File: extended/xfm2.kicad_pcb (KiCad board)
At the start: 2 copper layers, 69.2 x 121.3 mm, 32 parts, among them J1 Midi In, J2 Pin Breakout, J3 Midi Out, J4 Midi Thru, J5 Conn_Coaxial, U1 H11L1, U2 CmodA7-35T, U3 24LC01, U4 UDA1334A, U5 74HC14

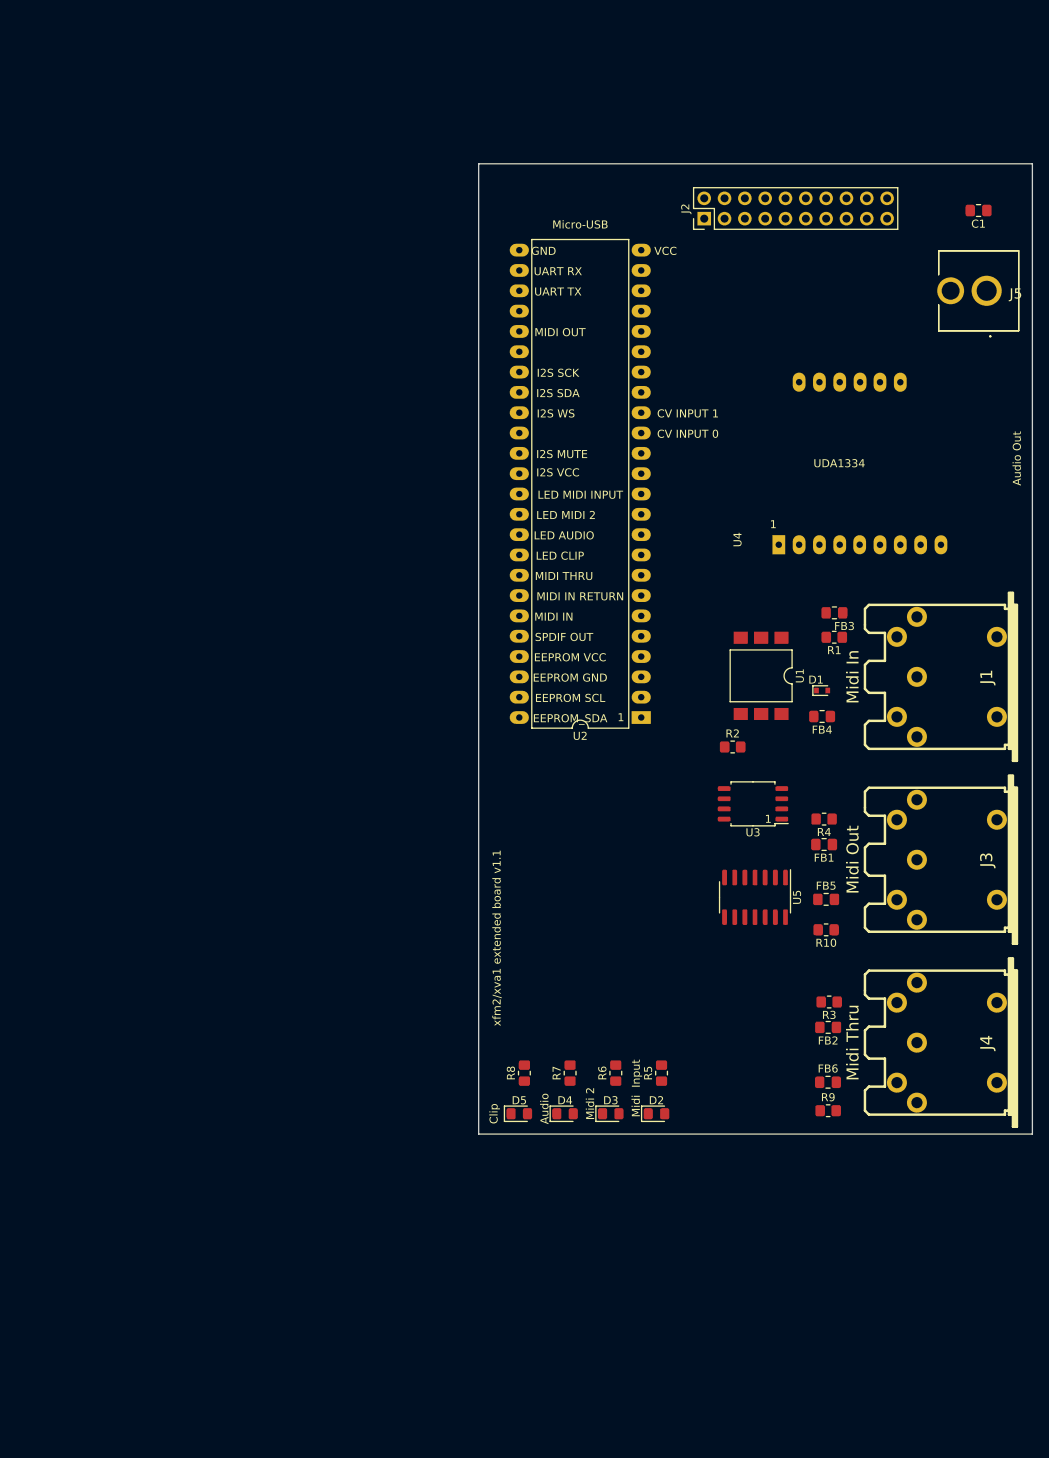
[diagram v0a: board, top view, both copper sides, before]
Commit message: initial extended pcb 1.1 placement
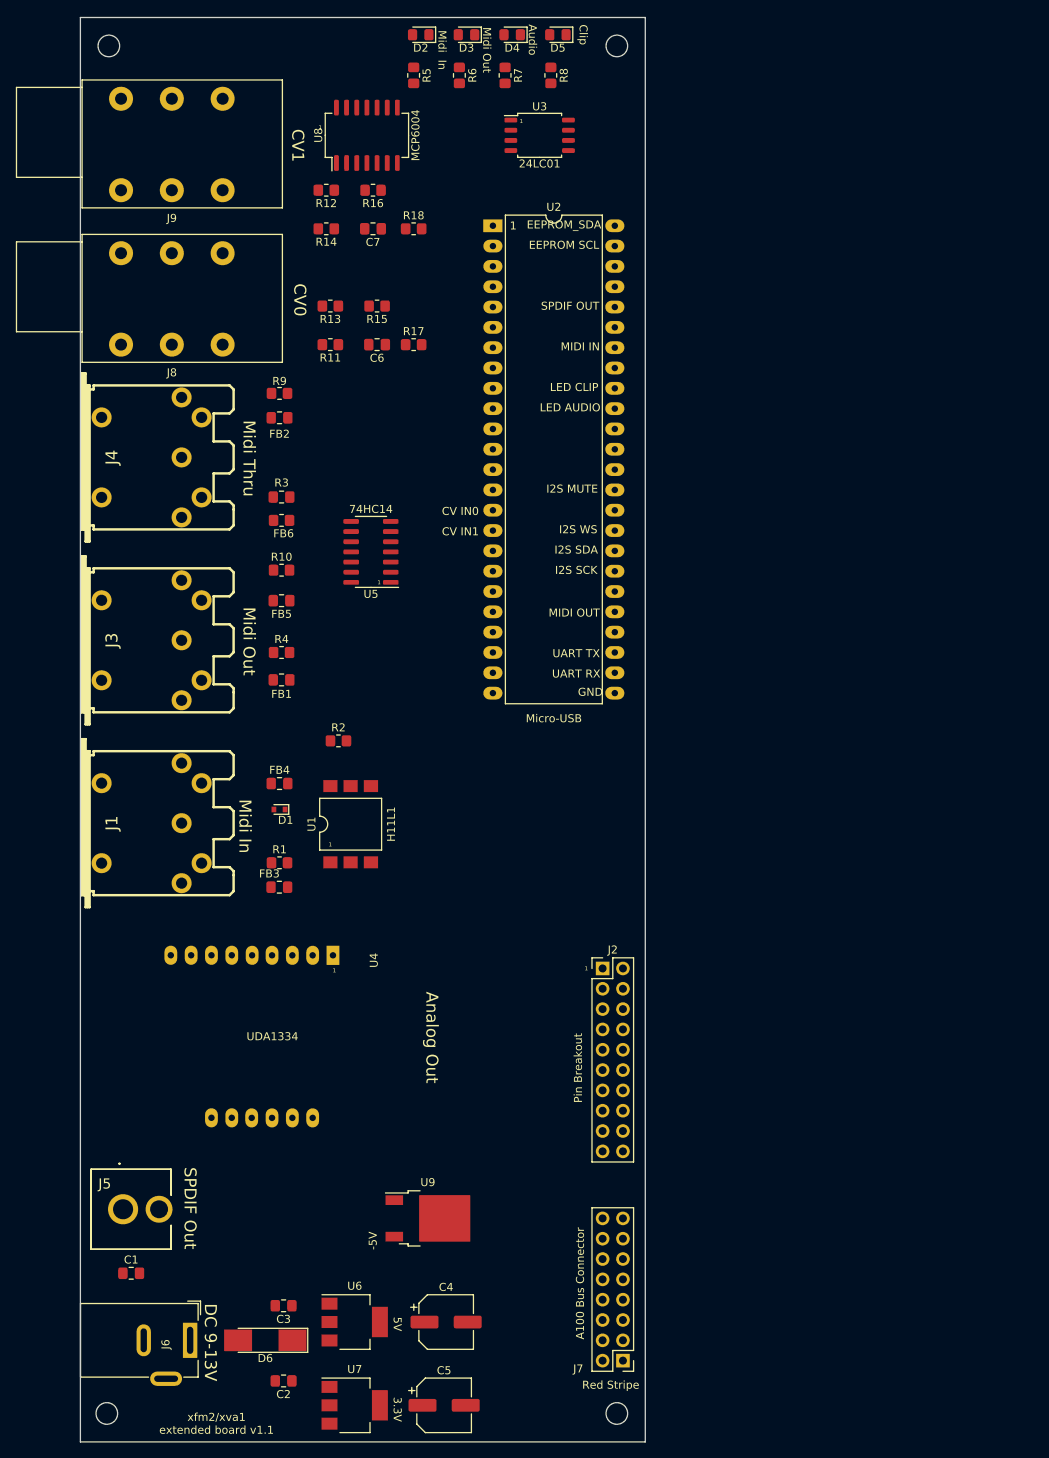
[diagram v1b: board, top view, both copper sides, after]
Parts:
- added C2: 10uF, Capacitor_SMD:C_0805_2012Metric_Pad1.18x1.45mm_HandSolder, F.Cu at (111.5, 186.4)
- added C3: 10uF, Capacitor_SMD:C_0805_2012Metric_Pad1.18x1.45mm_HandSolder, F.Cu at (111.5, 177.0)
- added C4: 100uF, Capacitor_SMD:CP_Elec_6.3x5.7, F.Cu at (131.8, 179.1)
- added C5: 100uF, Capacitor_SMD:CP_Elec_6.3x5.7, F.Cu at (131.6, 189.5)
- added C6: 330p-560p, Capacitor_SMD:C_0805_2012Metric_Pad1.18x1.45mm_HandSolder, F.Cu at (123.2, 56.9)
- added C7: 330p-560p, Capacitor_SMD:C_0805_2012Metric_Pad1.18x1.45mm_HandSolder, F.Cu at (122.7, 42.4)
- added D6: 1N4007, Diode_SMD:D_MELF_Handsoldering, F.Cu at (109.2, 181.4)
- added J6: Jack-DC, Connector_BarrelJack:BarrelJack_Wuerth_6941xx301002, F.Cu at (99.8, 181.4)
- added J7: A-100_Bus_Connector, Connector_PinHeader_2.54mm:PinHeader_2x08_P2.54mm_Vertical, F.Cu at (153.9, 183.9)
- added J8: AudioJack2, Connector_Audio:Jack_6.35mm_Neutrik_NRJ6HM-1_Horizontal, F.Cu at (103.9, 56.9)
- added J9: AudioJack2, Connector_Audio:Jack_6.35mm_Neutrik_NRJ6HM-1_Horizontal, F.Cu at (103.9, 37.6)
- added R11: 100k, Resistor_SMD:R_0805_2012Metric_Pad1.20x1.40mm_HandSolder, F.Cu at (117.3, 56.9)
- added R12: 100k, Resistor_SMD:R_0805_2012Metric_Pad1.20x1.40mm_HandSolder, F.Cu at (116.8, 37.6)
- added R13: 100k, Resistor_SMD:R_0805_2012Metric_Pad1.20x1.40mm_HandSolder, F.Cu at (117.3, 52.1)
- added R14: 100k, Resistor_SMD:R_0805_2012Metric_Pad1.20x1.40mm_HandSolder, F.Cu at (116.8, 42.4)
- added R15: 33k, Resistor_SMD:R_0805_2012Metric_Pad1.20x1.40mm_HandSolder, F.Cu at (123.2, 52.1)
- added R16: 33k, Resistor_SMD:R_0805_2012Metric_Pad1.20x1.40mm_HandSolder, F.Cu at (122.7, 37.6)
- added R17: 100, Resistor_SMD:R_0805_2012Metric_Pad1.20x1.40mm_HandSolder, F.Cu at (127.8, 56.9)
- added R18: 100, Resistor_SMD:R_0805_2012Metric_Pad1.20x1.40mm_HandSolder, F.Cu at (127.8, 42.4)
- added REF**: , MountingHole:MountingHole_2.7mm_M2.5, F.Cu at (89.7, 19.6)
- added REF**: , MountingHole:MountingHole_2.7mm_M2.5, F.Cu at (153.2, 19.6)
- added REF**: , MountingHole:MountingHole_2.7mm_M2.5, F.Cu at (153.2, 190.5)
- added REF**: , MountingHole:MountingHole_2.7mm_M2.5, F.Cu at (89.4, 190.5)
- added U6: LM1117-5.0, Package_TO_SOT_SMD:SOT-223-3_TabPin2, F.Cu at (120.4, 179.1)
- added U7: LM1117-3.3, Package_TO_SOT_SMD:SOT-223-3_TabPin2, F.Cu at (120.4, 189.5)
- added U8: MCP6004, Package_SO:SO-14_5.3x10.2mm_P1.27mm, F.Cu at (121.9, 30.7)
- added U9: MC79M05_TO252, Package_TO_SOT_SMD:TO-252-2, F.Cu at (129.5, 166.1)
- moved C1 169.9 mm to (92.5, 173.0), turned to 0 degrees
- moved J5 157.6 mm to (91.4, 165.0), turned to 0 degrees
- moved D2 138.1 mm to (128.7, 18.2), turned to 180 degrees
- moved D3 136.1 mm to (134.4, 18.2), turned to 180 degrees
- moved D4 135.0 mm to (140.1, 18.2), turned to 180 degrees
- moved D5 135.0 mm to (145.8, 18.2), turned to 180 degrees
- moved R5 128.5 mm to (127.8, 23.2), turned to 270 degrees
- moved R6 126.2 mm to (133.5, 23.2), turned to 270 degrees
- moved R7 125.0 mm to (139.2, 23.2), turned to 270 degrees
- moved R8 124.8 mm to (144.9, 23.2), turned to 270 degrees
- moved J4 122.2 mm to (95.8, 71.0), turned to 270 degrees
- moved R9 112.9 mm to (111.0, 63.0), turned to 180 degrees
- moved FB2 102.5 mm to (111.0, 66.0), turned to 0 degrees
- moved J3 101.7 mm to (95.8, 93.9), turned to 270 degrees
- moved FB6 100.1 mm to (111.3, 75.9), turned to 180 degrees
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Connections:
- J2 pad 10: I2S_VCC -> Net-(J2-Pad10)
- J2 pad 18: Net-(J2-Pad18) -> -5V
- J2 pad 19: Net-(J2-Pad19) -> +5V
- J2 pad 20: VCC -> +3V3
- R2 pad 1: EEPROM_VCC -> +3V3
- R3 pad 1: I2S_VCC -> +3V3
- R4 pad 2: I2S_VCC -> +3V3
- U1 pad 6: I2S_VCC -> +3V3
- U2 pad 15: Net-(U2-Pad15) -> CV0_3.3V
- U2 pad 16: Net-(U2-Pad16) -> CV1_3.3V
- U2 pad 24: VCC -> +5V
- U2 pad 36: I2S_VCC -> Net-(U2-Pad36)
- U2 pad 45: EEPROM_VCC -> Net-(U2-Pad45)
- U3 pad 3: EEPROM_VCC -> +3V3
- U3 pad 8: EEPROM_VCC -> +3V3
- U4 pad 1: I2S_VCC -> +3V3
- U4 pad 11: I2S_VCC -> +3V3
- U4 pad 13: I2S_VCC -> +3V3
- U5 pad 14: I2S_VCC -> +3V3
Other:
- board size 69.2 x 121.3 mm -> 70.6 x 178.1 mm
- board text added: "-5V"
- board text added: "24LC01"
- board text added: "3.3V"
- board text added: "5V"
- board text added: "74HC14"
- board text added: "A100 Bus Connector"
- board text added: "Analog Out"
- board text added: "CV IN0"
- board text added: "CV IN1"
- board text added: "CV0"
- board text added: "CV1"
- board text added: "DC 9-13V"
- board text added: "H11L1"
- board text added: "MCP6004"
- board text added: "Midi In"
- board text added: "Midi Out"
- board text added: "Midi Thru"
- board text added: "Pin Breakout"
- board text added: "Red Stripe"
- board text added: "SPDIF Out"
- board text removed: "Audio Out"
- board text removed: "CV INPUT 0"
- board text removed: "CV INPUT 1"
- board text removed: "EEPROM GND"
- board text removed: "EEPROM VCC"
- board text removed: "I2S VCC"
- board text removed: "LED MIDI 2"
- board text removed: "LED MIDI INPUT"
- board text removed: "MIDI IN RETURN"
- board text removed: "MIDI THRU"
- board text removed: "Midi 2"
- board text removed: "Midi Input"
- board text removed: "VCC"
